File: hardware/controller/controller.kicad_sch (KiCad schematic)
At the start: 8 parts, among them U1 ZX-PM2.54-1-16PY, U2 ZX-PM2.54-1-16PY, U3 ZX-PM2.54-1-16PY, U4 ZX-PM2.54-1-16PY

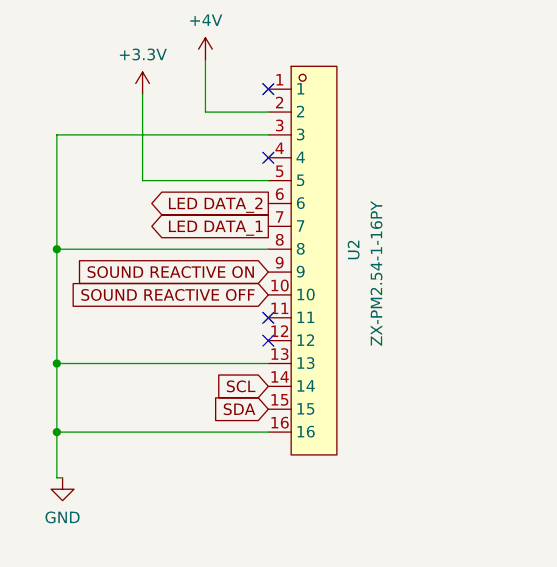
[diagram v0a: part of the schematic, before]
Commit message: cleanup and prep for ordering
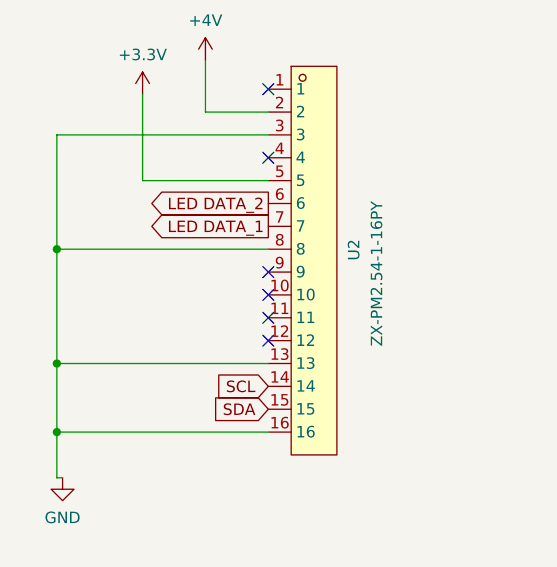
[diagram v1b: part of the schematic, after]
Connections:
- net SOUND REACTIVE OFF: no longer names the net of U2.10
- net SOUND REACTIVE ON: no longer names the net of U2.9
- no-connect marks 31 -> 33
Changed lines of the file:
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@@
+	)
+	(no_connect
+		(at 95.25 137.16)
 	)
 	(no_connect
@@
 	(no_connect
 		(at 161.29 57.15)
+	)
+	(no_connect
+		(at 95.25 134.62)
 	)
 	(no_connect
@@
 		)
 	)
-	(global_label "SOUND REACTIVE ON"
-		(shape input)
-		(at 95.25 134.62 180)
-		(fields_autoplaced yes)
-		(effects
-			(font
-				(size 1.27 1.27)
-			)
-			(justify right)
-		)
-		(property "Intersheetrefs" "${INTERSHEET_REFS}"
-			(at 72.61 134.62 0)
-			(hide yes)
-			(show_name no)
-			(do_not_autoplace no)
-			(effects
-				(font
-					(size 1.27 1.27)
-				)
-				(justify right)
-			)
-		)
-	)
 	(global_label "EAR TO EYE AUDIO"
 		(shape input)
@@
 			(hide yes)
 			(show_name no)
-			(do_not_autoplace no)
-			(effects
-				(font
-					(size 1.27 1.27)
-				)
-				(justify right)
-			)
-		)
-	)
-	(global_label "SOUND REACTIVE OFF"
-		(shape input)
-		(at 95.25 137.16 180)
-		(fields_autoplaced yes)
-		(effects
-			(font
-				(size 1.27 1.27)
-			)
-			(justify right)
-		)
-		(property "Intersheetrefs" "${INTERSHEET_REFS}"
-			(at 71.7633 137.16 0)
-			(hide yes)
-			(show_name no)
